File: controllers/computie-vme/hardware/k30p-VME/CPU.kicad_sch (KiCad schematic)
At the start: 15 parts, among them SW1 ~{RESET}, U1 MC68030RC, U2 74HC14, U3 74HC05

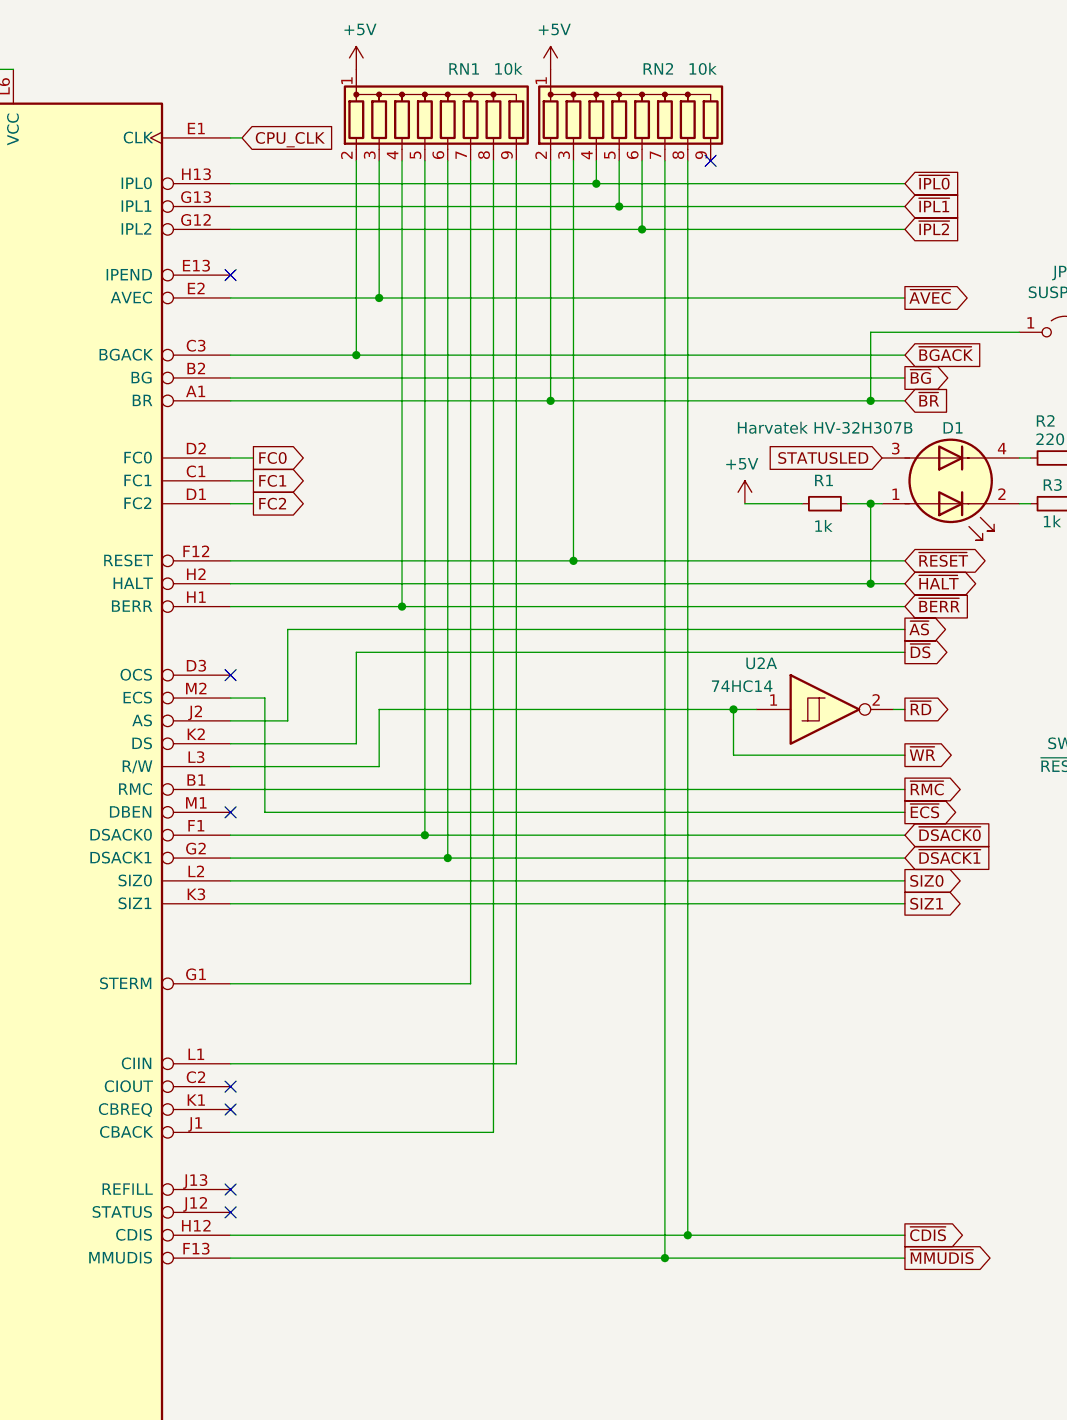
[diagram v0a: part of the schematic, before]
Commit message: k30p-VME PCB work in progress
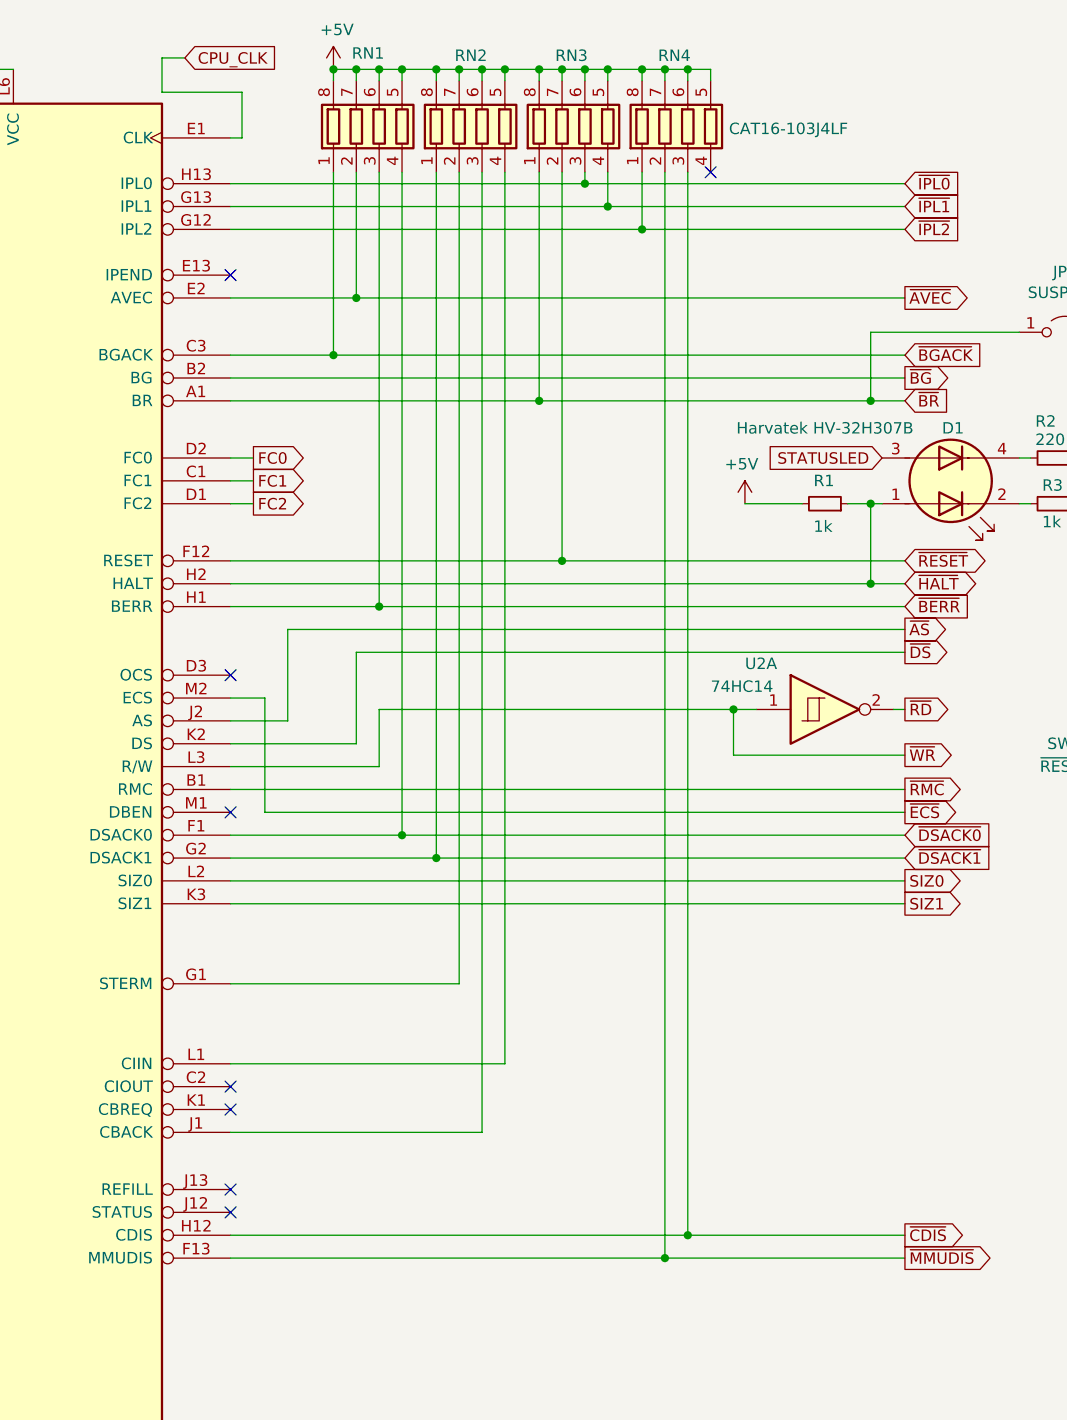
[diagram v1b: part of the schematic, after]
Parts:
- removed RN1, RN2: 10k, Resistor_THT:R_Array_SIP9, symbol Device:R_Network08
- added RN1, RN2, RN3, RN4: CAT16-103J4LF, Resistor_SMD:R_Cat16-4, symbol Device:R_Pack04
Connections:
- net +5V: now also RN1.5 (R4.2), RN1.6 (R3.2), RN1.7 (R2.2), RN1.8 (R1.2), RN2.5 (R4.2), RN2.6 (R3.2), RN2.7 (R2.2), RN2.8 (R1.2), RN3.5 (R4.2), RN3.6 (R3.2), RN3.7 (R2.2), RN3.8 (R1.2), RN4.5 (R4.2), RN4.6 (R3.2), RN4.7 (R2.2), RN4.8 (R1.2)
- net ~{AVEC}: now also RN1.2 (R2.1)
- net ~{BERR}: now also RN1.3 (R3.1)
- net ~{BGACK}: now also RN1.1 (R1.1)
- net ~{BR}: now also RN3.1 (R1.1)
- net ~{CDIS}: now also RN4.3 (R3.1)
- net ~{DSACK0}: now also RN1.4 (R4.1)
- net ~{DSACK1}: now also RN2.1 (R1.1)
- net ~{IPL0}: now also RN3.3 (R3.1)
- net ~{IPL1}: now also RN3.4 (R4.1)
- net ~{IPL2}: now also RN4.1 (R1.1)
- net ~{MMUDIS}: now also RN4.2 (R2.1)
- net ~{RESET}: now also RN3.2 (R2.1)
- net at U1.G1 (STERM): now also RN2.2 (R2.1)
- net at U1.J1 (CBACK): now also RN2.3 (R3.1)
- net at U1.L1 (CIIN): now also RN2.4 (R4.1)
